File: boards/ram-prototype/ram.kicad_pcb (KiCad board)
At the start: 4 copper layers, 200 x 52 mm, 391 parts, among them J1 PinHeader_1x16_P2.54mm_Vertic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, U1 DSBGA\-5_NumericPads, U10 DSBGA\-5_NumericPads, U100 DSBGA\-5_NumericPads, U101 DSBGA\-5_NumericPads, U102 DSBGA\-5_NumericPads, U103 DSBGA\-5_NumericPads, U104 DSBGA\-5_NumericPads, U105 DSBGA\-5_NumericPads, U106 DSBGA\-5_NumericPads, U107 DSBGA\-5_NumericPads, U108 DSBGA\-5_NumericPads, U109 DSBGA\-5_NumericPads, U11 DSBGA\-5_NumericPads, U110 DSBGA\-5_NumericPads, U111 DSBGA\-5_NumericPads, U112 DSBGA\-5_NumericPads, U113 DSBGA\-5_NumericPads, U114 DSBGA\-5_NumericPads, U115 DSBGA\-5_NumericPads, U116 DSBGA\-5_NumericPads, U117 DSBGA\-5_NumericPads, U118 DSBGA\-5_NumericPads, U119 DSBGA\-5_NumericPads, U12 DSBGA\-5_NumericPads, U120 DSBGA\-5_NumericPads, U121 DSBGA\-5_NumericPads, U122 DSBGA\-5_NumericPads, U123 DSBGA\-5_NumericPads, U124 DSBGA\-5_NumericPads, U125 DSBGA\-5_NumericPads, U126 DSBGA\-5_NumericPads, U127 DSBGA\-5_NumericPads, U128 DSBGA\-5_NumericPads, U129 DSBGA\-5_NumericPads, U13 DSBGA\-5_NumericPads, U130 DSBGA\-5_NumericPads, U131 DSBGA\-5_NumericPads, U132 DSBGA\-5_NumericPads, U133 DSBGA\-5_NumericPads, U134 DSBGA\-5_NumericPads, U135 DSBGA\-5_NumericPads, U136 DSBGA\-5_NumericPads, U137 DSBGA\-5_NumericPads, U138 DSBGA\-5_NumericPads, U139 DSBGA\-5_NumericPads, U14 DSBGA\-5_NumericPads, U140 DSBGA\-5_NumericPads, U141 DSBGA\-5_NumericPads, U142 DSBGA\-5_NumericPads, U143 DSBGA\-5_NumericPads, U144 DSBGA\-5_NumericPads, U145 DSBGA\-5_NumericPads, U146 DSBGA\-5_NumericPads, U147 DSBGA\-5_NumericPads, U148 DSBGA\-5_NumericPads, U149 DSBGA\-5_NumericPads, U15 DSBGA\-5_NumericPads, U150 DSBGA\-5_NumericPads, U151 DSBGA\-5_NumericPads, U152 DSBGA\-5_NumericPads, U153 DSBGA\-5_NumericPads, U154 DSBGA\-5_NumericPads, U155 DSBGA\-5_NumericPads, U156 DSBGA\-5_NumericPads, U157 DSBGA\-5_NumericPads, U158 DSBGA\-5_NumericPads, U16 DSBGA\-5_NumericPads, U17 DSBGA\-5_NumericPads, U18 DSBGA\-5_NumericPads, U19 DSBGA\-5_NumericPads, U2 DSBGA\-5_NumericPads, U20 DSBGA\-5_NumericPads, U21 DSBGA\-5_NumericPads, U22 DSBGA\-5_NumericPads, U23 DSBGA\-8_NumericPads, U24 DSBGA\-8_NumericPads, U25 DSBGA\-8_NumericPads, U26 DSBGA\-8_NumericPads, U27 DSBGA\-8_NumericPads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

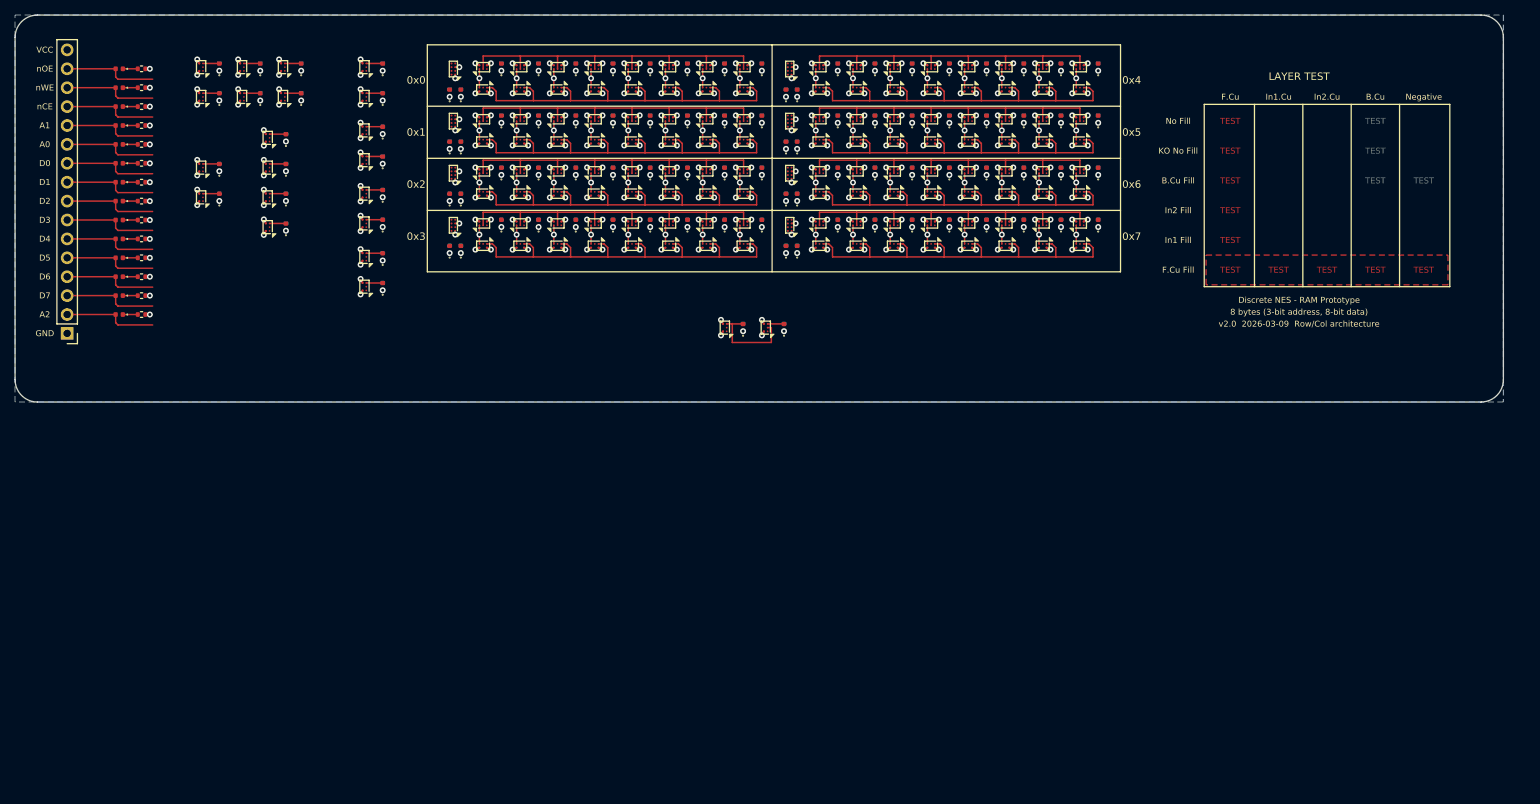
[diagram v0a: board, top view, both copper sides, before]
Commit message: Add initial changes to make logic close to final
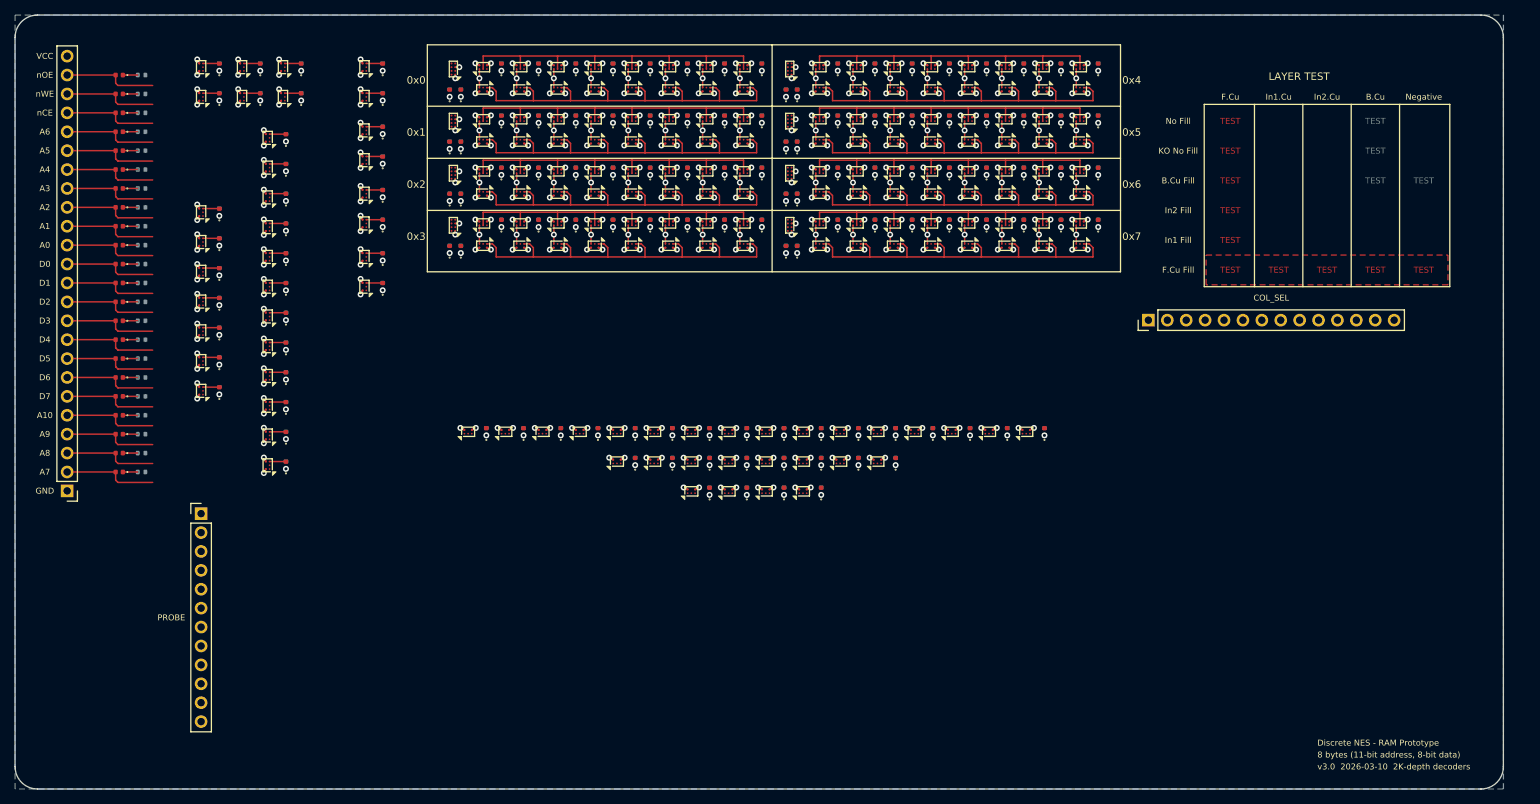
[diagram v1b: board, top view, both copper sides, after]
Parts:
- added D117: LED_0402_1005Metric, LED_SMD:LED_0402_1005Metric, F.Cu at (103.3, 27.0)
- added D118: LED_0402_1005Metric, LED_SMD:LED_0402_1005Metric, F.Cu at (103.3, 34.0)
- added D119: LED_0402_1005Metric, LED_SMD:LED_0402_1005Metric, F.Cu at (103.3, 41.0)
- added D120: LED_0402_1005Metric, LED_SMD:LED_0402_1005Metric, F.Cu at (148.6, 20.0)
- added D121: LED_0402_1005Metric, LED_SMD:LED_0402_1005Metric, F.Cu at (148.6, 27.0)
- added D122: LED_0402_1005Metric, LED_SMD:LED_0402_1005Metric, F.Cu at (148.6, 34.0)
- added D123: LED_0402_1005Metric, LED_SMD:LED_0402_1005Metric, F.Cu at (148.6, 41.0)
- added D124: LED_0402_1005Metric, LED_SMD:LED_0402_1005Metric, F.Cu at (98.3, 20.0)
- added D125: LED_0402_1005Metric, LED_SMD:LED_0402_1005Metric, F.Cu at (98.3, 27.0)
- added D126: LED_0402_1005Metric, LED_SMD:LED_0402_1005Metric, F.Cu at (98.3, 34.0)
- added D127: LED_0402_1005Metric, LED_SMD:LED_0402_1005Metric, F.Cu at (98.3, 41.0)
- added D128: LED_0402_1005Metric, LED_SMD:LED_0402_1005Metric, F.Cu at (143.6, 20.0)
- added D129: LED_0402_1005Metric, LED_SMD:LED_0402_1005Metric, F.Cu at (143.6, 27.0)
- added D130: LED_0402_1005Metric, LED_SMD:LED_0402_1005Metric, F.Cu at (143.6, 34.0)
- added D131: LED_0402_1005Metric, LED_SMD:LED_0402_1005Metric, F.Cu at (143.6, 41.0)
- added D132: LED_0402_1005Metric, LED_SMD:LED_0402_1005Metric, F.Cu at (93.3, 20.0)
- added D133: LED_0402_1005Metric, LED_SMD:LED_0402_1005Metric, F.Cu at (93.3, 27.0)
- added D134: LED_0402_1005Metric, LED_SMD:LED_0402_1005Metric, F.Cu at (93.3, 34.0)
- added D135: LED_0402_1005Metric, LED_SMD:LED_0402_1005Metric, F.Cu at (93.3, 41.0)
- added D136: LED_0402_1005Metric, LED_SMD:LED_0402_1005Metric, F.Cu at (138.6, 20.0)
- added D137: LED_0402_1005Metric, LED_SMD:LED_0402_1005Metric, F.Cu at (138.6, 27.0)
- added D138: LED_0402_1005Metric, LED_SMD:LED_0402_1005Metric, F.Cu at (138.6, 34.0)
- added D139: LED_0402_1005Metric, LED_SMD:LED_0402_1005Metric, F.Cu at (138.6, 41.0)
- added D140: LED_0402_1005Metric, LED_SMD:LED_0402_1005Metric, F.Cu at (88.3, 20.0)
- added D141: LED_0402_1005Metric, LED_SMD:LED_0402_1005Metric, F.Cu at (88.3, 27.0)
- added D142: LED_0402_1005Metric, LED_SMD:LED_0402_1005Metric, F.Cu at (88.3, 34.0)
- added D143: LED_0402_1005Metric, LED_SMD:LED_0402_1005Metric, F.Cu at (88.3, 41.0)
- added D144: LED_0402_1005Metric, LED_SMD:LED_0402_1005Metric, F.Cu at (133.6, 20.0)
- added D145: LED_0402_1005Metric, LED_SMD:LED_0402_1005Metric, F.Cu at (133.6, 27.0)
- added D146: LED_0402_1005Metric, LED_SMD:LED_0402_1005Metric, F.Cu at (133.6, 34.0)
- added D147: LED_0402_1005Metric, LED_SMD:LED_0402_1005Metric, F.Cu at (133.6, 41.0)
- added D148: LED_0402_1005Metric, LED_SMD:LED_0402_1005Metric, F.Cu at (83.3, 20.0)
- added D149: LED_0402_1005Metric, LED_SMD:LED_0402_1005Metric, F.Cu at (83.3, 27.0)
- added D150: LED_0402_1005Metric, LED_SMD:LED_0402_1005Metric, F.Cu at (83.3, 34.0)
- added D151: LED_0402_1005Metric, LED_SMD:LED_0402_1005Metric, F.Cu at (83.3, 41.0)
- added D152: LED_0402_1005Metric, LED_SMD:LED_0402_1005Metric, F.Cu at (128.6, 20.0)
- added D153: LED_0402_1005Metric, LED_SMD:LED_0402_1005Metric, F.Cu at (128.6, 27.0)
- added D154: LED_0402_1005Metric, LED_SMD:LED_0402_1005Metric, F.Cu at (128.6, 34.0)
- added D155: LED_0402_1005Metric, LED_SMD:LED_0402_1005Metric, F.Cu at (128.6, 41.0)
- added D156: LED_0402_1005Metric, LED_SMD:LED_0402_1005Metric, F.Cu at (78.3, 20.0)
- added D157: LED_0402_1005Metric, LED_SMD:LED_0402_1005Metric, F.Cu at (78.3, 27.0)
- added D158: LED_0402_1005Metric, LED_SMD:LED_0402_1005Metric, F.Cu at (78.3, 34.0)
- added D159: LED_0402_1005Metric, LED_SMD:LED_0402_1005Metric, F.Cu at (78.3, 41.0)
- added D160: LED_0402_1005Metric, LED_SMD:LED_0402_1005Metric, F.Cu at (123.5, 20.0)
- added D161: LED_0402_1005Metric, LED_SMD:LED_0402_1005Metric, F.Cu at (123.5, 27.0)
- added D162: LED_0402_1005Metric, LED_SMD:LED_0402_1005Metric, F.Cu at (123.5, 34.0)
- added D163: LED_0402_1005Metric, LED_SMD:LED_0402_1005Metric, F.Cu at (123.5, 41.0)
- added J2: PinHeader_1x12_P2.54mm_Vertical, Connector_PinHeader_2.54mm:PinHeader_1x12_P2.54mm_Vertical, B.Cu at (38.0, 80.0)
- added J3: PinHeader_1x14_P2.54mm_Vertical, Connector_PinHeader_2.54mm:PinHeader_1x14_P2.54mm_Vertical, B.Cu at (165.3, 54.0)
- added R117: R_0402_1005Metric, Resistor_SMD:R_0402_1005Metric, B.Cu at (103.3, 27.0)
- added R118: R_0402_1005Metric, Resistor_SMD:R_0402_1005Metric, B.Cu at (103.3, 34.0)
- added R119: R_0402_1005Metric, Resistor_SMD:R_0402_1005Metric, B.Cu at (103.3, 41.0)
- added R120: R_0402_1005Metric, Resistor_SMD:R_0402_1005Metric, B.Cu at (148.6, 20.0)
- added R121: R_0402_1005Metric, Resistor_SMD:R_0402_1005Metric, B.Cu at (148.6, 27.0)
- added R122: R_0402_1005Metric, Resistor_SMD:R_0402_1005Metric, B.Cu at (148.6, 34.0)
- added R123: R_0402_1005Metric, Resistor_SMD:R_0402_1005Metric, B.Cu at (148.6, 41.0)
- added R124: R_0402_1005Metric, Resistor_SMD:R_0402_1005Metric, B.Cu at (98.3, 20.0)
- added R125: R_0402_1005Metric, Resistor_SMD:R_0402_1005Metric, B.Cu at (98.3, 27.0)
- added R126: R_0402_1005Metric, Resistor_SMD:R_0402_1005Metric, B.Cu at (98.3, 34.0)
- added R127: R_0402_1005Metric, Resistor_SMD:R_0402_1005Metric, B.Cu at (98.3, 41.0)
- added R128: R_0402_1005Metric, Resistor_SMD:R_0402_1005Metric, B.Cu at (143.6, 20.0)
- added R129: R_0402_1005Metric, Resistor_SMD:R_0402_1005Metric, B.Cu at (143.6, 27.0)
- added R130: R_0402_1005Metric, Resistor_SMD:R_0402_1005Metric, B.Cu at (143.6, 34.0)
- added R131: R_0402_1005Metric, Resistor_SMD:R_0402_1005Metric, B.Cu at (143.6, 41.0)
- added R132: R_0402_1005Metric, Resistor_SMD:R_0402_1005Metric, B.Cu at (93.3, 20.0)
- added R133: R_0402_1005Metric, Resistor_SMD:R_0402_1005Metric, B.Cu at (93.3, 27.0)
- added R134: R_0402_1005Metric, Resistor_SMD:R_0402_1005Metric, B.Cu at (93.3, 34.0)
- added R135: R_0402_1005Metric, Resistor_SMD:R_0402_1005Metric, B.Cu at (93.3, 41.0)
- added R136: R_0402_1005Metric, Resistor_SMD:R_0402_1005Metric, B.Cu at (138.6, 20.0)
- added R137: R_0402_1005Metric, Resistor_SMD:R_0402_1005Metric, B.Cu at (138.6, 27.0)
- added R138: R_0402_1005Metric, Resistor_SMD:R_0402_1005Metric, B.Cu at (138.6, 34.0)
- added R139: R_0402_1005Metric, Resistor_SMD:R_0402_1005Metric, B.Cu at (138.6, 41.0)
- added R140: R_0402_1005Metric, Resistor_SMD:R_0402_1005Metric, B.Cu at (88.3, 20.0)
- added R141: R_0402_1005Metric, Resistor_SMD:R_0402_1005Metric, B.Cu at (88.3, 27.0)
- added R142: R_0402_1005Metric, Resistor_SMD:R_0402_1005Metric, B.Cu at (88.3, 34.0)
- added R143: R_0402_1005Metric, Resistor_SMD:R_0402_1005Metric, B.Cu at (88.3, 41.0)
- added R144: R_0402_1005Metric, Resistor_SMD:R_0402_1005Metric, B.Cu at (133.6, 20.0)
- added R145: R_0402_1005Metric, Resistor_SMD:R_0402_1005Metric, B.Cu at (133.6, 27.0)
- added R146: R_0402_1005Metric, Resistor_SMD:R_0402_1005Metric, B.Cu at (133.6, 34.0)
- added R147: R_0402_1005Metric, Resistor_SMD:R_0402_1005Metric, B.Cu at (133.6, 41.0)
- added R148: R_0402_1005Metric, Resistor_SMD:R_0402_1005Metric, B.Cu at (83.3, 20.0)
- added R149: R_0402_1005Metric, Resistor_SMD:R_0402_1005Metric, B.Cu at (83.3, 27.0)
- added R150: R_0402_1005Metric, Resistor_SMD:R_0402_1005Metric, B.Cu at (83.3, 34.0)
- added R151: R_0402_1005Metric, Resistor_SMD:R_0402_1005Metric, B.Cu at (83.3, 41.0)
- added R152: R_0402_1005Metric, Resistor_SMD:R_0402_1005Metric, B.Cu at (128.6, 20.0)
- added R153: R_0402_1005Metric, Resistor_SMD:R_0402_1005Metric, B.Cu at (128.6, 27.0)
- added R154: R_0402_1005Metric, Resistor_SMD:R_0402_1005Metric, B.Cu at (128.6, 34.0)
- added R155: R_0402_1005Metric, Resistor_SMD:R_0402_1005Metric, B.Cu at (128.6, 41.0)
- added R156: R_0402_1005Metric, Resistor_SMD:R_0402_1005Metric, B.Cu at (78.3, 20.0)
- added R157: R_0402_1005Metric, Resistor_SMD:R_0402_1005Metric, B.Cu at (78.3, 27.0)
- added R158: R_0402_1005Metric, Resistor_SMD:R_0402_1005Metric, B.Cu at (78.3, 34.0)
- added R159: R_0402_1005Metric, Resistor_SMD:R_0402_1005Metric, B.Cu at (78.3, 41.0)
- added R160: R_0402_1005Metric, Resistor_SMD:R_0402_1005Metric, B.Cu at (123.5, 20.0)
- added R161: R_0402_1005Metric, Resistor_SMD:R_0402_1005Metric, B.Cu at (123.5, 27.0)
- added R162: R_0402_1005Metric, Resistor_SMD:R_0402_1005Metric, B.Cu at (123.5, 34.0)
- added R163: R_0402_1005Metric, Resistor_SMD:R_0402_1005Metric, B.Cu at (123.5, 41.0)
- added U159: DSBGA\-5_NumericPads, DSBGA_Packages:DSBGA-5_NumericPads, F.Cu at (85.9, 30.0)
- added U160: DSBGA\-5_NumericPads, DSBGA_Packages:DSBGA-5_NumericPads, F.Cu at (85.9, 37.0)
- added U161: DSBGA\-5_NumericPads, DSBGA_Packages:DSBGA-5_NumericPads, F.Cu at (85.9, 44.0)
- added U162: DSBGA\-5_NumericPads, DSBGA_Packages:DSBGA-5_NumericPads, F.Cu at (131.1, 23.0)
- added U163: DSBGA\-5_NumericPads, DSBGA_Packages:DSBGA-5_NumericPads, F.Cu at (131.1, 30.0)
- added U164: DSBGA\-5_NumericPads, DSBGA_Packages:DSBGA-5_NumericPads, F.Cu at (131.1, 37.0)
- added U165: DSBGA\-5_NumericPads, DSBGA_Packages:DSBGA-5_NumericPads, F.Cu at (131.1, 44.0)
- added U166: DSBGA\-5_NumericPads, DSBGA_Packages:DSBGA-5_NumericPads, F.Cu at (80.9, 20.0)
- added U167: DSBGA\-5_NumericPads, DSBGA_Packages:DSBGA-5_NumericPads, F.Cu at (80.9, 27.0)
- added U168: DSBGA\-5_NumericPads, DSBGA_Packages:DSBGA-5_NumericPads, F.Cu at (80.9, 34.0)
- added U169: DSBGA\-5_NumericPads, DSBGA_Packages:DSBGA-5_NumericPads, F.Cu at (80.9, 41.0)
- added U170: DSBGA\-5_NumericPads, DSBGA_Packages:DSBGA-5_NumericPads, F.Cu at (126.1, 20.0)
- added U171: DSBGA\-5_NumericPads, DSBGA_Packages:DSBGA-5_NumericPads, F.Cu at (126.1, 27.0)
- added U172: DSBGA\-5_NumericPads, DSBGA_Packages:DSBGA-5_NumericPads, F.Cu at (126.1, 34.0)
- added U173: DSBGA\-5_NumericPads, DSBGA_Packages:DSBGA-5_NumericPads, F.Cu at (126.1, 41.0)
- added U174: DSBGA\-5_NumericPads, DSBGA_Packages:DSBGA-5_NumericPads, F.Cu at (80.9, 23.0)
- added U175: DSBGA\-5_NumericPads, DSBGA_Packages:DSBGA-5_NumericPads, F.Cu at (80.9, 30.0)
- added U176: DSBGA\-5_NumericPads, DSBGA_Packages:DSBGA-5_NumericPads, F.Cu at (80.9, 37.0)
- added U177: DSBGA\-5_NumericPads, DSBGA_Packages:DSBGA-5_NumericPads, F.Cu at (80.9, 44.0)
- added U178: DSBGA\-5_NumericPads, DSBGA_Packages:DSBGA-5_NumericPads, F.Cu at (126.1, 23.0)
- added U179: DSBGA\-5_NumericPads, DSBGA_Packages:DSBGA-5_NumericPads, F.Cu at (126.1, 30.0)
- added U180: DSBGA\-5_NumericPads, DSBGA_Packages:DSBGA-5_NumericPads, F.Cu at (126.1, 37.0)
- added U181: DSBGA\-5_NumericPads, DSBGA_Packages:DSBGA-5_NumericPads, F.Cu at (126.1, 44.0)
- added U182: DSBGA\-5_NumericPads, DSBGA_Packages:DSBGA-5_NumericPads, F.Cu at (75.9, 20.0)
- added U183: DSBGA\-5_NumericPads, DSBGA_Packages:DSBGA-5_NumericPads, F.Cu at (75.9, 27.0)
- added U184: DSBGA\-5_NumericPads, DSBGA_Packages:DSBGA-5_NumericPads, F.Cu at (75.9, 34.0)
- added U185: DSBGA\-5_NumericPads, DSBGA_Packages:DSBGA-5_NumericPads, F.Cu at (75.9, 41.0)
- added U186: DSBGA\-5_NumericPads, DSBGA_Packages:DSBGA-5_NumericPads, F.Cu at (121.1, 20.0)
- added U187: DSBGA\-5_NumericPads, DSBGA_Packages:DSBGA-5_NumericPads, F.Cu at (121.1, 27.0)
- added U188: DSBGA\-5_NumericPads, DSBGA_Packages:DSBGA-5_NumericPads, F.Cu at (121.1, 34.0)
- added U189: DSBGA\-5_NumericPads, DSBGA_Packages:DSBGA-5_NumericPads, F.Cu at (121.1, 41.0)
- added U190: DSBGA\-5_NumericPads, DSBGA_Packages:DSBGA-5_NumericPads, F.Cu at (75.9, 23.0)
- added U191: DSBGA\-5_NumericPads, DSBGA_Packages:DSBGA-5_NumericPads, F.Cu at (75.9, 30.0)
- added U192: DSBGA\-5_NumericPads, DSBGA_Packages:DSBGA-5_NumericPads, F.Cu at (75.9, 37.0)
- added U193: DSBGA\-5_NumericPads, DSBGA_Packages:DSBGA-5_NumericPads, F.Cu at (75.9, 44.0)
- added U194: DSBGA\-5_NumericPads, DSBGA_Packages:DSBGA-5_NumericPads, F.Cu at (121.1, 23.0)
- added U195: DSBGA\-5_NumericPads, DSBGA_Packages:DSBGA-5_NumericPads, F.Cu at (121.1, 30.0)
- added U196: DSBGA\-5_NumericPads, DSBGA_Packages:DSBGA-5_NumericPads, F.Cu at (121.1, 37.0)
- added U197: DSBGA\-5_NumericPads, DSBGA_Packages:DSBGA-5_NumericPads, F.Cu at (121.1, 44.0)
- J1: value PinHeader_1x16_P2.54mm_Vertical -> PinHeader_1x24_P2.54mm_Vertical; footprint Connector_PinHeader_2.54mm:PinHeader_1x16_P2.54mm_Vertical -> Connector_PinHeader_2.54mm:PinHeader_1x24_P2.54mm_Vertical
- R1, R10, R11, R12, R13, R14, R2, R3, R4, R5, R6, R7, R8, R9: moved to B.Cu
- U23, U24, U25, U26, U27, U28, U29, U30: value DSBGA\-8_NumericPads -> DSBGA\-5_NumericPads; footprint DSBGA_Packages:DSBGA-8_NumericPads -> DSBGA_Packages:DSBGA-5_NumericPads
- U62, U63, U64, U65, U66, U67, U68, U69: value DSBGA\-5_NumericPads -> DSBGA\-8_NumericPads; footprint DSBGA_Packages:DSBGA-5_NumericPads -> DSBGA_Packages:DSBGA-8_NumericPads
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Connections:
- D10 pad 2: /D4 -> /Address Decoder/A0
- D11 pad 2: /D5 -> /D0
- D12 pad 2: /D6 -> /D1
- D13 pad 2: /D7 -> /D2
- D14 pad 2: /Column Select/A2 -> /D3
- D15 pad 2: Net-(D15-A) -> /D4
- D16 pad 2: Net-(D16-A) -> /D5
- D17 pad 2: /Address Decoder/ROW_SEL_0 -> /D6
- D18 pad 2: /Address Decoder/ROW_SEL_1 -> /D7
- D19 pad 2: /Address Decoder/ROW_SEL_2 -> /Column Select/A10
- D20 pad 2: /Address Decoder/ROW_SEL_3 -> /Column Select/A9
- D21 pad 2: /COL_SEL_0 -> /Column Select/A8
- D22 pad 2: /COL_SEL_1 -> /Column Select/A7
- D27 pad 2: /WRITE_ACTIVE -> Net-(D27-A)
- D28 pad 2: /READ_EN -> Net-(D28-A)
- D29 pad 2: /WRITE_EN_ROW_0 -> Net-(D29-A)
- D30 pad 2: /WRITE_EN_ROW_1 -> /RS1
- D31 pad 2: /WRITE_EN_ROW_2 -> /RS2
- D32 pad 2: /WRITE_EN_ROW_3 -> /RS3
- D33 pad 2: /READ_EN_ROW_0 -> /RS4
- D34 pad 2: /READ_EN_ROW_1 -> Net-(D34-A)
- D35 pad 2: /READ_EN_ROW_2 -> Net-(D35-A)
- D36 pad 2: /READ_EN_ROW_3 -> Net-(D36-A)
- D38 pad 2: Net-(D38-A) -> /Address Decoder/ROW_SEL_0
- D39 pad 2: Net-(D39-A) -> /Address Decoder/ROW_SEL_1
- D4 pad 2: /Address Decoder/A1 -> /Address Decoder/A6
- D40 pad 2: Net-(D40-A) -> /Address Decoder/ROW_SEL_2
- D41 pad 2: Net-(D41-A) -> /Address Decoder/ROW_SEL_3
- D46 pad 2: Net-(D46-A) -> /GA0
- D47 pad 2: Net-(D47-A) -> /GA1
- D48 pad 2: Net-(D48-A) -> /GA2
- D49 pad 2: Net-(D49-A) -> /GA3
- D5 pad 2: /Address Decoder/A0 -> /Address Decoder/A5
- D50 pad 2: Net-(D50-A) -> /GB0
- D51 pad 2: Net-(D51-A) -> /GB1
- D52 pad 2: Net-(D52-A) -> /GB2
- D53 pad 2: Net-(D53-A) -> /GB3
- D54 pad 2: Net-(D54-A) -> /COL_SEL_0
- D55 pad 2: Net-(D55-A) -> /COL_SEL_1
- D56 pad 2: Net-(D56-A) -> /COL_SEL_2
- D57 pad 2: Net-(D57-A) -> /COL_SEL_3
- D58 pad 2: Net-(D58-A) -> /COL_SEL_4
- D59 pad 2: Net-(D59-A) -> /COL_SEL_5
- D6 pad 2: /D0 -> /Address Decoder/A4
- D60 pad 2: Net-(D60-A) -> /COL_SEL_6
- D61 pad 2: Net-(D61-A) -> /COL_SEL_7
- D62 pad 2: Net-(D62-A) -> /COL_SEL_8
- D63 pad 2: Net-(D63-A) -> /COL_SEL_9
- D64 pad 2: Net-(D64-A) -> /COL_SEL_10
- D65 pad 2: Net-(D65-A) -> /COL_SEL_11
- D66 pad 2: Net-(D66-A) -> /COL_SEL_12
- D67 pad 2: Net-(D67-A) -> /COL_SEL_13
- D68 pad 2: Net-(D68-A) -> /COL_SEL_14
- D69 pad 2: Net-(D69-A) -> /COL_SEL_15
- D7 pad 2: /D1 -> /Address Decoder/A3
- D74 pad 2: Net-(D74-A) -> /WRITE_ACTIVE
- D75 pad 2: Net-(D75-A) -> /READ_EN
- D76 pad 2: Net-(D76-A) -> /WRITE_EN_ROW_0
- D77 pad 2: Net-(D77-A) -> /WRITE_EN_ROW_1
- D78 pad 2: Net-(D78-A) -> /WRITE_EN_ROW_2
- D79 pad 2: Net-(D79-A) -> /WRITE_EN_ROW_3
- D8 pad 2: /D2 -> /Address Decoder/A2
- D80 pad 2: Net-(D80-A) -> /READ_EN_ROW_0
- D81 pad 2: Net-(D81-A) -> /READ_EN_ROW_1
- D82 pad 2: Net-(D82-A) -> /READ_EN_ROW_2
- D83 pad 2: Net-(D83-A) -> /READ_EN_ROW_3
- D9 pad 2: /D3 -> /Address Decoder/A1
- J1 pad 10: /D0 -> /D3
- J1 pad 11: /Address Decoder/A0 -> /D2
- J1 pad 12: /Address Decoder/A1 -> /D1
- J1 pad 13: /Control Logic/nCE -> /D0
- J1 pad 14: /Control Logic/nWE -> /Address Decoder/A0
- J1 pad 15: /Control Logic/nOE -> /Address Decoder/A1
- J1 pad 16: VCC -> /Address Decoder/A2
- J1 pad 2: /Column Select/A2 -> /Column Select/A7
- J1 pad 3: /D7 -> /Column Select/A8
- J1 pad 4: /D6 -> /Column Select/A9
- J1 pad 5: /D5 -> /Column Select/A10
- J1 pad 6: /D4 -> /D7
- J1 pad 7: /D3 -> /D6
- J1 pad 8: /D2 -> /D5
- J1 pad 9: /D1 -> /D4
- U1 pad 4: Net-(D15-A) -> Net-(D23-A)
- U10 pad 1: (no net) -> /RS1
- U10 pad 2: /Control Logic/nOE -> /RS2
- U10 pad 4: Net-(D24-A) -> /RS3
- U100 pad 1: /D4 -> Net-(D98-A)
- U100 pad 2: Net-(D42-A) -> Net-(D114-A)
- U100 pad 4: Net-(D90-A) -> /D1
- U101 pad 1: /D4 -> Net-(D99-A)
- U101 pad 2: Net-(D43-A) -> Net-(D115-A)
- U101 pad 4: Net-(D91-A) -> /D1
- U102 pad 1: /D4 -> /D2
- U102 pad 2: Net-(D44-A) -> Net-(D84-A)
- U102 pad 4: Net-(D92-A) -> Net-(D116-A)
- U103 pad 1: Net-(D45-A) -> /D2
- U103 pad 4: /D4 -> Net-(D117-A)
- U104 pad 1: Net-(D46-A) -> /D2
- U104 pad 4: /D4 -> Net-(D118-A)
- U105 pad 1: Net-(D47-A) -> /D2
- U105 pad 4: /D4 -> Net-(D119-A)
- U106 pad 1: Net-(D48-A) -> /D2
- U106 pad 4: /D4 -> Net-(D120-A)
- U107 pad 1: Net-(D49-A) -> /D2
- U107 pad 4: /D4 -> Net-(D121-A)
- U108 pad 1: Net-(D50-A) -> /D2
- U108 pad 4: /D4 -> Net-(D122-A)
- U109 pad 1: Net-(D51-A) -> /D2
- U109 pad 4: /D4 -> Net-(D123-A)
- U11 pad 1: (no net) -> /RS3
- U11 pad 2: /Control Logic/nWE -> Net-(D29-A)
- U11 pad 4: Net-(D25-A) -> /RS4
- U110 pad 1: Net-(D52-A) -> Net-(D92-A)
- U110 pad 2: Net-(D92-A) -> Net-(D116-A)
- U110 pad 4: /D4 -> /D2
- U111 pad 1: /D5 -> Net-(D93-A)
- U111 pad 2: Net-(D37-A) -> Net-(D117-A)
- U111 pad 4: Net-(D93-A) -> /D2
- U112 pad 1: /D5 -> Net-(D94-A)
- U112 pad 2: Net-(D38-A) -> Net-(D118-A)
- U112 pad 4: Net-(D94-A) -> /D2
- U113 pad 1: /D5 -> Net-(D95-A)
- U113 pad 2: Net-(D39-A) -> Net-(D119-A)
- U113 pad 4: Net-(D95-A) -> /D2
- U114 pad 1: /D5 -> Net-(D96-A)
- U114 pad 2: Net-(D40-A) -> Net-(D120-A)
- U114 pad 4: Net-(D96-A) -> /D2
- U115 pad 1: /D5 -> Net-(D97-A)
- U115 pad 2: Net-(D41-A) -> Net-(D121-A)
- U115 pad 4: Net-(D97-A) -> /D2
- U116 pad 1: /D5 -> Net-(D98-A)
- U116 pad 2: Net-(D42-A) -> Net-(D122-A)
- U116 pad 4: Net-(D98-A) -> /D2
- U117 pad 1: /D5 -> Net-(D99-A)
- U117 pad 2: Net-(D43-A) -> Net-(D123-A)
- U117 pad 4: Net-(D99-A) -> /D2
- U118 pad 1: /D5 -> /D3
- U118 pad 2: Net-(D44-A) -> Net-(D84-A)
- U118 pad 4: Net-(D100-A) -> Net-(D124-A)
- U119 pad 1: Net-(D45-A) -> /D3
- U119 pad 2: Net-(D93-A) -> Net-(D85-A)
- U119 pad 4: /D5 -> Net-(D125-A)
- U12 pad 1: Net-(D23-A) -> Net-(D24-A)
- U12 pad 2: Net-(D25-A) -> Net-(D23-A)
- U12 pad 4: /WRITE_ACTIVE -> Net-(D34-A)
- U120 pad 1: Net-(D46-A) -> /D3
- U120 pad 2: Net-(D94-A) -> Net-(D86-A)
- U120 pad 4: /D5 -> Net-(D126-A)
- U121 pad 1: Net-(D47-A) -> /D3
- U121 pad 2: Net-(D95-A) -> Net-(D87-A)
- U121 pad 4: /D5 -> Net-(D127-A)
- U122 pad 1: Net-(D48-A) -> /D3
- U122 pad 2: Net-(D96-A) -> Net-(D88-A)
- U122 pad 4: /D5 -> Net-(D128-A)
- U123 pad 1: Net-(D49-A) -> /D3
- U123 pad 2: Net-(D97-A) -> Net-(D89-A)
- U123 pad 4: /D5 -> Net-(D129-A)
- U124 pad 1: Net-(D50-A) -> /D3
- U124 pad 2: Net-(D98-A) -> Net-(D90-A)
- U124 pad 4: /D5 -> Net-(D130-A)
- U125 pad 1: Net-(D51-A) -> /D3
- U125 pad 2: Net-(D99-A) -> Net-(D91-A)
- U125 pad 4: /D5 -> Net-(D131-A)
- U126 pad 1: Net-(D52-A) -> Net-(D92-A)
- U126 pad 2: Net-(D100-A) -> Net-(D124-A)
- U126 pad 4: /D5 -> /D3
- U127 pad 1: /D6 -> Net-(D93-A)
- U127 pad 2: Net-(D37-A) -> Net-(D125-A)
- U127 pad 4: Net-(D101-A) -> /D3
- U128 pad 1: /D6 -> Net-(D94-A)
- U128 pad 2: Net-(D38-A) -> Net-(D126-A)
- U128 pad 4: Net-(D102-A) -> /D3
- U129 pad 1: /D6 -> Net-(D95-A)
- U129 pad 2: Net-(D39-A) -> Net-(D127-A)
- U129 pad 4: Net-(D103-A) -> /D3
- U13 pad 1: Net-(D23-A) -> Net-(D24-A)
- U13 pad 2: Net-(D24-A) -> /Address Decoder/A0
- U13 pad 4: Net-(D26-A) -> Net-(D35-A)
- U130 pad 1: /D6 -> Net-(D96-A)
- U130 pad 2: Net-(D40-A) -> Net-(D128-A)
- U130 pad 4: Net-(D104-A) -> /D3
- U131 pad 1: /D6 -> Net-(D97-A)
- U131 pad 2: Net-(D41-A) -> Net-(D129-A)
- U131 pad 4: Net-(D105-A) -> /D3
- U132 pad 1: /D6 -> Net-(D98-A)
- U132 pad 2: Net-(D42-A) -> Net-(D130-A)
- U132 pad 4: Net-(D106-A) -> /D3
- U133 pad 1: /D6 -> Net-(D99-A)
- U133 pad 2: Net-(D43-A) -> Net-(D131-A)
- U133 pad 4: Net-(D107-A) -> /D3
- U134 pad 1: /D6 -> /D4
- U134 pad 2: Net-(D44-A) -> Net-(D84-A)
- U134 pad 4: Net-(D108-A) -> Net-(D132-A)
- U135 pad 1: Net-(D45-A) -> /D4
- U135 pad 2: Net-(D101-A) -> Net-(D85-A)
- U135 pad 4: /D6 -> Net-(D133-A)
- U136 pad 1: Net-(D46-A) -> /D4
- U136 pad 2: Net-(D102-A) -> Net-(D86-A)
- U136 pad 4: /D6 -> Net-(D134-A)
- U137 pad 1: Net-(D47-A) -> /D4
- U137 pad 2: Net-(D103-A) -> Net-(D87-A)
- U137 pad 4: /D6 -> Net-(D135-A)
- U138 pad 1: Net-(D48-A) -> /D4
- U138 pad 2: Net-(D104-A) -> Net-(D88-A)
- U138 pad 4: /D6 -> Net-(D136-A)
- U139 pad 1: Net-(D49-A) -> /D4
- U139 pad 2: Net-(D105-A) -> Net-(D89-A)
- U139 pad 4: /D6 -> Net-(D137-A)
- U14 pad 1: Net-(D26-A) -> /Address Decoder/A1
- U14 pad 2: /Control Logic/nWE -> Net-(D23-A)
- U14 pad 4: /READ_EN -> Net-(D36-A)
- U140 pad 1: Net-(D50-A) -> /D4
- U140 pad 2: Net-(D106-A) -> Net-(D90-A)
- U140 pad 4: /D6 -> Net-(D138-A)
- U141 pad 1: Net-(D51-A) -> /D4
- U141 pad 2: Net-(D107-A) -> Net-(D91-A)
- U141 pad 4: /D6 -> Net-(D139-A)
- U142 pad 1: Net-(D52-A) -> Net-(D92-A)
- U142 pad 2: Net-(D108-A) -> Net-(D132-A)
- U142 pad 4: /D6 -> /D4
- U143 pad 1: /D7 -> Net-(D93-A)
- U143 pad 2: Net-(D37-A) -> Net-(D133-A)
- U143 pad 4: Net-(D109-A) -> /D4
- U144 pad 1: /D7 -> Net-(D94-A)
- U144 pad 2: Net-(D38-A) -> Net-(D134-A)
- U144 pad 4: Net-(D110-A) -> /D4
- U145 pad 1: /D7 -> Net-(D95-A)
- U145 pad 2: Net-(D39-A) -> Net-(D135-A)
- U145 pad 4: Net-(D111-A) -> /D4
- U146 pad 1: /D7 -> Net-(D96-A)
- U146 pad 2: Net-(D40-A) -> Net-(D136-A)
- U146 pad 4: Net-(D112-A) -> /D4
- U147 pad 1: /D7 -> Net-(D97-A)
- U147 pad 2: Net-(D41-A) -> Net-(D137-A)
- U147 pad 4: Net-(D113-A) -> /D4
- U148 pad 1: /D7 -> Net-(D98-A)
- U148 pad 2: Net-(D42-A) -> Net-(D138-A)
- U148 pad 4: Net-(D114-A) -> /D4
- U149 pad 1: /D7 -> Net-(D99-A)
- U149 pad 2: Net-(D43-A) -> Net-(D139-A)
- U149 pad 4: Net-(D115-A) -> /D4
- U15 pad 1: /WRITE_ACTIVE -> /Address Decoder/A1
- U15 pad 2: /Address Decoder/ROW_SEL_0 -> /Address Decoder/A0
- U15 pad 4: /WRITE_EN_ROW_0 -> Net-(D37-A)
- U150 pad 1: /D7 -> /D5
- U150 pad 2: Net-(D44-A) -> Net-(D84-A)
- U150 pad 4: Net-(D116-A) -> Net-(D140-A)
- U151 pad 1: Net-(D45-A) -> /D5
- U151 pad 2: Net-(D109-A) -> Net-(D85-A)
- U151 pad 4: /D7 -> Net-(D141-A)
- U152 pad 1: Net-(D46-A) -> /D5
- U152 pad 2: Net-(D110-A) -> Net-(D86-A)
- U152 pad 4: /D7 -> Net-(D142-A)
- U153 pad 1: Net-(D47-A) -> /D5
- U153 pad 2: Net-(D111-A) -> Net-(D87-A)
- U153 pad 4: /D7 -> Net-(D143-A)
- U154 pad 1: Net-(D48-A) -> /D5
- U154 pad 2: Net-(D112-A) -> Net-(D88-A)
- U154 pad 4: /D7 -> Net-(D144-A)
- U155 pad 1: Net-(D49-A) -> /D5
- U155 pad 2: Net-(D113-A) -> Net-(D89-A)
- U155 pad 4: /D7 -> Net-(D145-A)
- U156 pad 1: Net-(D50-A) -> /D5
- U156 pad 2: Net-(D114-A) -> Net-(D90-A)
- U156 pad 4: /D7 -> Net-(D146-A)
- U157 pad 1: Net-(D51-A) -> /D5
- U157 pad 2: Net-(D115-A) -> Net-(D91-A)
- U157 pad 4: /D7 -> Net-(D147-A)
- U158 pad 1: Net-(D52-A) -> Net-(D92-A)
- U158 pad 2: Net-(D116-A) -> Net-(D140-A)
- U158 pad 4: /D7 -> /D5
- U16 pad 1: /WRITE_ACTIVE -> /RS4
- U16 pad 2: /Address Decoder/ROW_SEL_1 -> Net-(D34-A)
- U16 pad 4: /WRITE_EN_ROW_1 -> /Address Decoder/ROW_SEL_0
- U17 pad 1: /WRITE_ACTIVE -> /RS4
- U17 pad 2: /Address Decoder/ROW_SEL_2 -> Net-(D35-A)
- U17 pad 4: /WRITE_EN_ROW_2 -> /Address Decoder/ROW_SEL_1
- U18 pad 1: /WRITE_ACTIVE -> /RS4
- U18 pad 2: /Address Decoder/ROW_SEL_3 -> Net-(D36-A)
- U18 pad 4: /WRITE_EN_ROW_3 -> /Address Decoder/ROW_SEL_2
- U19 pad 1: /READ_EN -> /RS4
- U19 pad 2: /Address Decoder/ROW_SEL_0 -> Net-(D37-A)
- U19 pad 4: /READ_EN_ROW_0 -> /Address Decoder/ROW_SEL_3
- U2 pad 4: Net-(D16-A) -> Net-(D24-A)
- U20 pad 1: /READ_EN -> (no net)
- U20 pad 2: /Address Decoder/ROW_SEL_1 -> /Column Select/A7
- U20 pad 4: /READ_EN_ROW_1 -> Net-(D42-A)
- U21 pad 1: /READ_EN -> (no net)
- U21 pad 2: /Address Decoder/ROW_SEL_2 -> /Column Select/A8
- U21 pad 4: /READ_EN_ROW_2 -> Net-(D43-A)
- U22 pad 1: /READ_EN -> (no net)
- U22 pad 2: /Address Decoder/ROW_SEL_3 -> /Column Select/A9
- U22 pad 4: /READ_EN_ROW_3 -> Net-(D44-A)
- U23 pad 1: /COL_SEL_0 -> (no net)
- U23 pad 2: /WRITE_EN_ROW_0 -> /Column Select/A10
- U23 pad 3: Net-(D45-A) -> GND
- U23 pad 4: GND -> Net-(D45-A)
- U23 pad 5: /COL_SEL_0 -> VCC
- U24 pad 1: /COL_SEL_0 -> Net-(D43-A)
- U24 pad 2: /WRITE_EN_ROW_1 -> Net-(D42-A)
- U24 pad 3: Net-(D46-A) -> GND
- U24 pad 4: GND -> /GA0
- U24 pad 5: /COL_SEL_0 -> VCC
- U25 pad 1: /COL_SEL_0 -> Net-(D43-A)
- U25 pad 2: /WRITE_EN_ROW_2 -> /Column Select/A7
- U25 pad 3: Net-(D47-A) -> GND
- U25 pad 4: GND -> /GA1
- U25 pad 5: /COL_SEL_0 -> VCC
- U26 pad 1: /COL_SEL_0 -> /Column Select/A8
- U26 pad 2: /WRITE_EN_ROW_3 -> Net-(D42-A)
- U26 pad 3: Net-(D48-A) -> GND
- U26 pad 4: GND -> /GA2
- U26 pad 5: /COL_SEL_0 -> VCC
- U27 pad 1: /COL_SEL_1 -> /Column Select/A8
- U27 pad 2: /WRITE_EN_ROW_0 -> /Column Select/A7
- U27 pad 3: Net-(D49-A) -> GND
- U27 pad 4: GND -> /GA3
- U27 pad 5: /COL_SEL_1 -> VCC
- U28 pad 1: /COL_SEL_1 -> Net-(D45-A)
- U28 pad 2: /WRITE_EN_ROW_1 -> Net-(D44-A)
- U28 pad 3: Net-(D50-A) -> GND
- U28 pad 4: GND -> /GB0
- U28 pad 5: /COL_SEL_1 -> VCC
- U29 pad 1: /COL_SEL_1 -> Net-(D45-A)
- U29 pad 2: /WRITE_EN_ROW_2 -> /Column Select/A9
- U29 pad 3: Net-(D51-A) -> GND
- U29 pad 4: GND -> /GB1
- U29 pad 5: /COL_SEL_1 -> VCC
- U3 pad 1: Net-(D15-A) -> (no net)
- U3 pad 2: Net-(D16-A) -> /Address Decoder/A2
- U3 pad 4: /Address Decoder/ROW_SEL_0 -> Net-(D25-A)
- U30 pad 1: /COL_SEL_1 -> /Column Select/A10
- U30 pad 2: /WRITE_EN_ROW_3 -> Net-(D44-A)
- U30 pad 3: Net-(D52-A) -> GND
- U30 pad 4: GND -> /GB2
- U30 pad 5: /COL_SEL_1 -> VCC
- U31 pad 1: /D0 -> /Column Select/A10
- U31 pad 2: Net-(D37-A) -> /Column Select/A9
- U31 pad 4: Net-(D53-A) -> /GB3
- U32 pad 1: /D0 -> /GB0
- U32 pad 2: Net-(D38-A) -> /GA0
- U32 pad 4: Net-(D54-A) -> /COL_SEL_0
- U33 pad 1: /D0 -> /GB0
- U33 pad 2: Net-(D39-A) -> /GA1
- U33 pad 4: Net-(D55-A) -> /COL_SEL_1
- U34 pad 1: /D0 -> /GB0
- U34 pad 2: Net-(D40-A) -> /GA2
- U34 pad 4: Net-(D56-A) -> /COL_SEL_2
- U35 pad 1: /D0 -> /GB0
- U35 pad 2: Net-(D41-A) -> /GA3
- U35 pad 4: Net-(D57-A) -> /COL_SEL_3
- U36 pad 1: /D0 -> /GB1
- U36 pad 2: Net-(D42-A) -> /GA0
- U36 pad 4: Net-(D58-A) -> /COL_SEL_4
- U37 pad 1: /D0 -> /GB1
- U37 pad 2: Net-(D43-A) -> /GA1
- U37 pad 4: Net-(D59-A) -> /COL_SEL_5
- U38 pad 1: /D0 -> /GB1
- U38 pad 2: Net-(D44-A) -> /GA2
- U38 pad 4: Net-(D60-A) -> /COL_SEL_6
- U39 pad 1: Net-(D45-A) -> /GB1
- U39 pad 2: Net-(D53-A) -> /GA3
- U39 pad 4: /D0 -> /COL_SEL_7
- U4 pad 1: /Address Decoder/A0 -> (no net)
- U4 pad 2: Net-(D16-A) -> /Address Decoder/A3
- U4 pad 4: /Address Decoder/ROW_SEL_1 -> Net-(D26-A)
- U40 pad 1: Net-(D46-A) -> /GB2
- U40 pad 2: Net-(D54-A) -> /GA0
- U40 pad 4: /D0 -> /COL_SEL_8
- U41 pad 1: Net-(D47-A) -> /GB2
- U41 pad 2: Net-(D55-A) -> /GA1
- U41 pad 4: /D0 -> /COL_SEL_9
- U42 pad 1: Net-(D48-A) -> /GB2
- U42 pad 2: Net-(D56-A) -> /GA2
- U42 pad 4: /D0 -> /COL_SEL_10
- U43 pad 1: Net-(D49-A) -> /GB2
- U43 pad 2: Net-(D57-A) -> /GA3
- U43 pad 4: /D0 -> /COL_SEL_11
- U44 pad 1: Net-(D50-A) -> /GB3
- U44 pad 2: Net-(D58-A) -> /GA0
- U44 pad 4: /D0 -> /COL_SEL_12
- U45 pad 1: Net-(D51-A) -> /GB3
- U45 pad 2: Net-(D59-A) -> /GA1
- U45 pad 4: /D0 -> /COL_SEL_13
- U46 pad 1: Net-(D52-A) -> /GB3
- U46 pad 2: Net-(D60-A) -> /GA2
- U46 pad 4: /D0 -> /COL_SEL_14
- U47 pad 1: /D1 -> /GB3
- U47 pad 2: Net-(D37-A) -> /GA3
- U47 pad 4: Net-(D61-A) -> /COL_SEL_15
- U48 pad 1: /D1 -> (no net)
- U48 pad 2: Net-(D38-A) -> /Control Logic/nCE
- U48 pad 4: Net-(D62-A) -> Net-(D70-A)
- U49 pad 1: /D1 -> (no net)
- U49 pad 2: Net-(D39-A) -> /Control Logic/nOE
- U49 pad 4: Net-(D63-A) -> Net-(D71-A)
- U5 pad 1: Net-(D15-A) -> (no net)
- U5 pad 2: /Address Decoder/A1 -> /Address Decoder/A4
- U5 pad 4: /Address Decoder/ROW_SEL_2 -> Net-(D27-A)
- U50 pad 1: /D1 -> (no net)
- U50 pad 2: Net-(D40-A) -> /Control Logic/nWE
- U50 pad 4: Net-(D64-A) -> Net-(D72-A)
- U51 pad 1: /D1 -> Net-(D70-A)
- U51 pad 2: Net-(D41-A) -> Net-(D72-A)
- U51 pad 4: Net-(D65-A) -> /WRITE_ACTIVE
- U52 pad 1: /D1 -> Net-(D70-A)
- U52 pad 2: Net-(D42-A) -> Net-(D71-A)
- U52 pad 4: Net-(D66-A) -> Net-(D73-A)
- U53 pad 1: /D1 -> Net-(D73-A)
- U53 pad 2: Net-(D43-A) -> /Control Logic/nWE
- U53 pad 4: Net-(D67-A) -> /READ_EN
- U54 pad 1: /D1 -> /WRITE_ACTIVE
- U54 pad 2: Net-(D44-A) -> /Address Decoder/ROW_SEL_0
- U54 pad 4: Net-(D68-A) -> /WRITE_EN_ROW_0
- U55 pad 1: Net-(D45-A) -> /WRITE_ACTIVE
- U55 pad 2: Net-(D61-A) -> /Address Decoder/ROW_SEL_1
- U55 pad 4: /D1 -> /WRITE_EN_ROW_1
- U56 pad 1: Net-(D46-A) -> /WRITE_ACTIVE
- U56 pad 2: Net-(D62-A) -> /Address Decoder/ROW_SEL_2
- U56 pad 4: /D1 -> /WRITE_EN_ROW_2
- U57 pad 1: Net-(D47-A) -> /WRITE_ACTIVE
- U57 pad 2: Net-(D63-A) -> /Address Decoder/ROW_SEL_3
- U57 pad 4: /D1 -> /WRITE_EN_ROW_3
- U58 pad 1: Net-(D48-A) -> /READ_EN
- U58 pad 2: Net-(D64-A) -> /Address Decoder/ROW_SEL_0
- U58 pad 4: /D1 -> /READ_EN_ROW_0
- U59 pad 1: Net-(D49-A) -> /READ_EN
- U59 pad 2: Net-(D65-A) -> /Address Decoder/ROW_SEL_1
- U59 pad 4: /D1 -> /READ_EN_ROW_1
- U6 pad 1: /Address Decoder/A0 -> (no net)
- U6 pad 2: /Address Decoder/A1 -> /Address Decoder/A5
- U6 pad 4: /Address Decoder/ROW_SEL_3 -> Net-(D28-A)
- U60 pad 1: Net-(D50-A) -> /READ_EN
- U60 pad 2: Net-(D66-A) -> /Address Decoder/ROW_SEL_2
- U60 pad 4: /D1 -> /READ_EN_ROW_2
- U61 pad 1: Net-(D51-A) -> /READ_EN
- U61 pad 2: Net-(D67-A) -> /Address Decoder/ROW_SEL_3
- U61 pad 4: /D1 -> /READ_EN_ROW_3
- U62 pad 1: Net-(D52-A) -> /COL_SEL_0
- U62 pad 2: Net-(D68-A) -> /WRITE_EN_ROW_0
- U62 pad 3: GND -> Net-(D92-A)
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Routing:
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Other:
- board size 200 x 52 mm -> 200 x 104 mm
- board text added: "8 bytes (11-bit address, 8-bit data)"
- board text added: "A10"
- board text added: "A3"
- board text added: "A4"
- board text added: "A5"
- board text added: "A6"
- board text added: "A7"
- board text added: "A8"
- board text added: "A9"
- board text added: "COL_SEL"
- board text added: "PROBE"
- board text added: "v3.0 2026-03-10 2K-depth decoders"
- board text removed: "8 bytes (3-bit address, 8-bit data)"
- board text removed: "v2.0 2026-03-09 Row/Col architecture"

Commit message: clean up
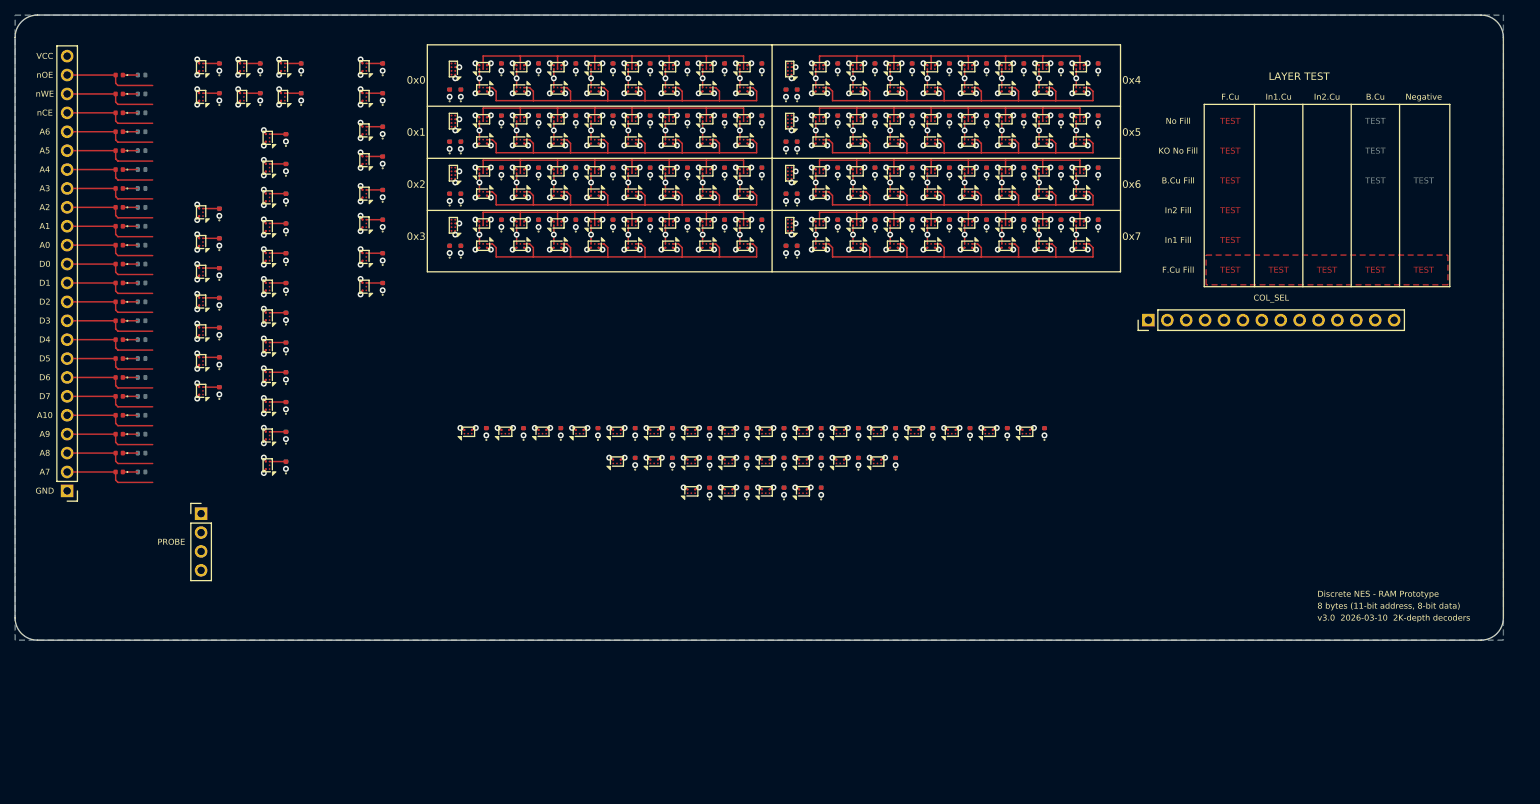
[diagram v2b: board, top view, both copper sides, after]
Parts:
- J2: value PinHeader_1x12_P2.54mm_Vertical -> PinHeader_1x04_P2.54mm_Vertical; footprint Connector_PinHeader_2.54mm:PinHeader_1x12_P2.54mm_Vertical -> Connector_PinHeader_2.54mm:PinHeader_1x04_P2.54mm_Vertical
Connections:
- D46 pad 2: /GA0 -> /Column Select/GA0
- D47 pad 2: /GA1 -> /Column Select/GA1
- D48 pad 2: /GA2 -> /Column Select/GA2
- D49 pad 2: /GA3 -> /Column Select/GA3
- D50 pad 2: /GB0 -> /Column Select/GB0
- D51 pad 2: /GB1 -> /Column Select/GB1
- D52 pad 2: /GB2 -> /Column Select/GB2
- D53 pad 2: /GB3 -> /Column Select/GB3
- U24 pad 4: /GA0 -> /Column Select/GA0
- U25 pad 4: /GA1 -> /Column Select/GA1
- U26 pad 4: /GA2 -> /Column Select/GA2
- U27 pad 4: /GA3 -> /Column Select/GA3
- U28 pad 4: /GB0 -> /Column Select/GB0
- U29 pad 4: /GB1 -> /Column Select/GB1
- U30 pad 4: /GB2 -> /Column Select/GB2
- U31 pad 4: /GB3 -> /Column Select/GB3
- U32 pad 1: /GB0 -> /Column Select/GB0
- U32 pad 2: /GA0 -> /Column Select/GA0
- U33 pad 1: /GB0 -> /Column Select/GB0
- U33 pad 2: /GA1 -> /Column Select/GA1
- U34 pad 1: /GB0 -> /Column Select/GB0
- U34 pad 2: /GA2 -> /Column Select/GA2
- U35 pad 1: /GB0 -> /Column Select/GB0
- U35 pad 2: /GA3 -> /Column Select/GA3
- U36 pad 1: /GB1 -> /Column Select/GB1
- U36 pad 2: /GA0 -> /Column Select/GA0
- U37 pad 1: /GB1 -> /Column Select/GB1
- U37 pad 2: /GA1 -> /Column Select/GA1
- U38 pad 1: /GB1 -> /Column Select/GB1
- U38 pad 2: /GA2 -> /Column Select/GA2
- U39 pad 1: /GB1 -> /Column Select/GB1
- U39 pad 2: /GA3 -> /Column Select/GA3
- U40 pad 1: /GB2 -> /Column Select/GB2
- U40 pad 2: /GA0 -> /Column Select/GA0
- U41 pad 1: /GB2 -> /Column Select/GB2
- U41 pad 2: /GA1 -> /Column Select/GA1
- U42 pad 1: /GB2 -> /Column Select/GB2
- U42 pad 2: /GA2 -> /Column Select/GA2
- U43 pad 1: /GB2 -> /Column Select/GB2
- U43 pad 2: /GA3 -> /Column Select/GA3
- U44 pad 1: /GB3 -> /Column Select/GB3
- U44 pad 2: /GA0 -> /Column Select/GA0
- U45 pad 1: /GB3 -> /Column Select/GB3
- U45 pad 2: /GA1 -> /Column Select/GA1
- U46 pad 1: /GB3 -> /Column Select/GB3
- U46 pad 2: /GA2 -> /Column Select/GA2
- U47 pad 1: /GB3 -> /Column Select/GB3
- U47 pad 2: /GA3 -> /Column Select/GA3
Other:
- board size 200 x 104 mm -> 200 x 84 mm
